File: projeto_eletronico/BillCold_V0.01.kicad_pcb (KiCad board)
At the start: 2 copper layers, 53 x 53 mm, 54 parts, among them J1 USB_B, SW1 SW_Push, SW2 SW_SPDT_321, U1 ESP32-S3, U2 AMS1117, U3 W25Q128JVSIQ, U4 USBLC6-2SC6, X1 OSCILADOR-3225

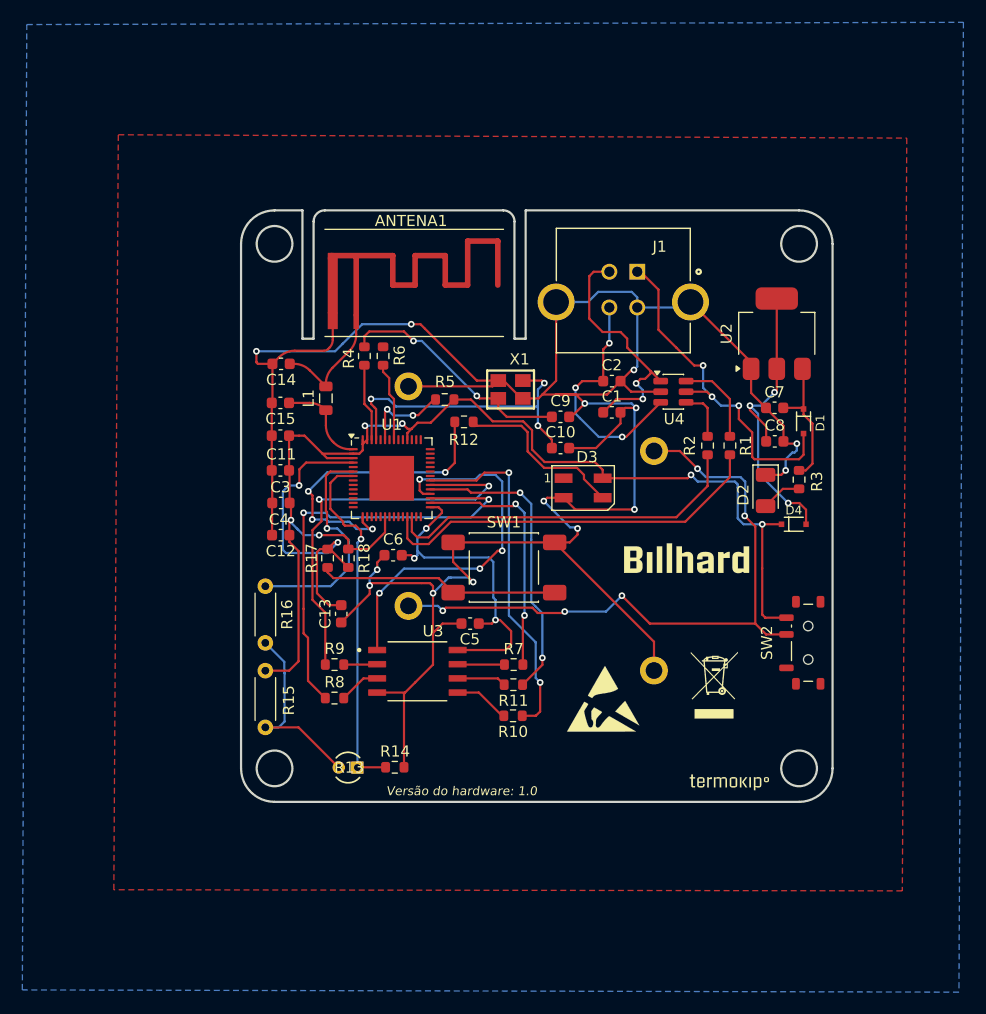
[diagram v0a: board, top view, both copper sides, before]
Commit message: Conclusão do projeto
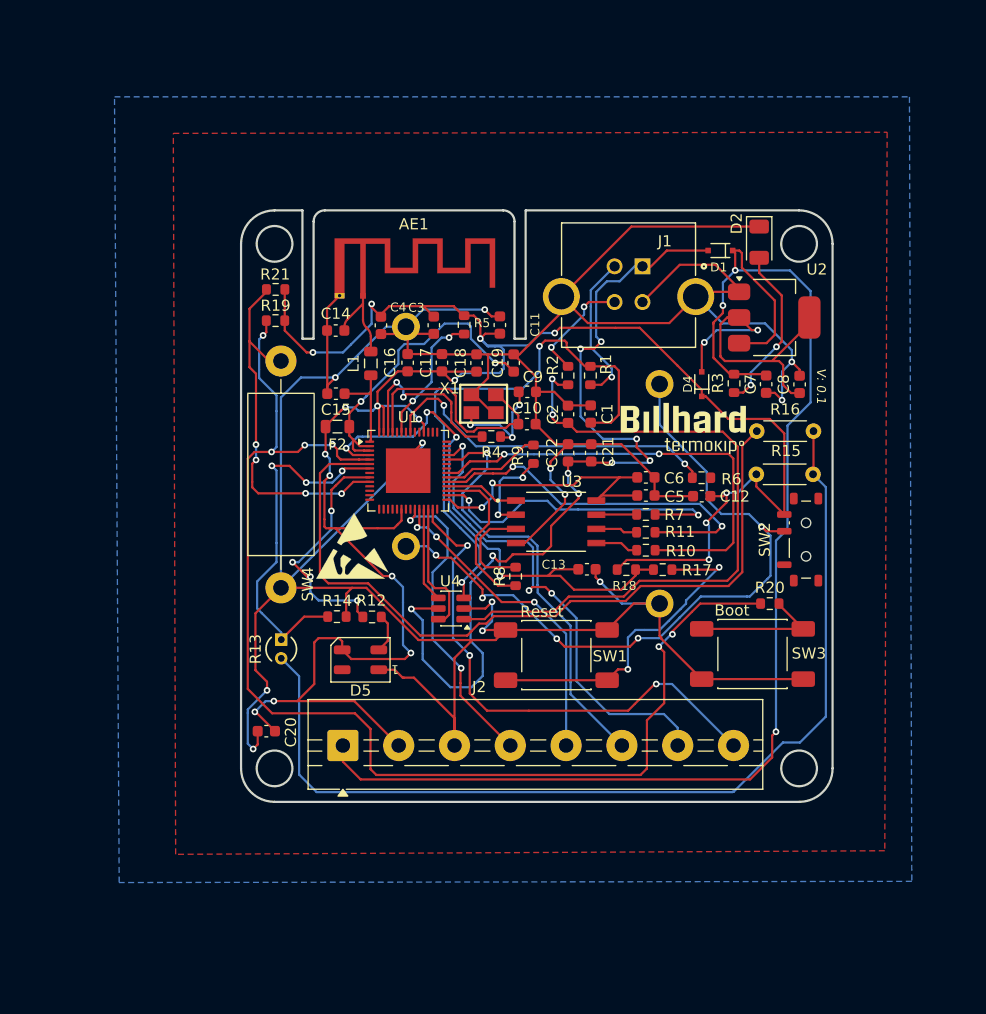
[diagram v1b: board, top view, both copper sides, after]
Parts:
- removed ANTENA1: ANT_2.4GB, ANTENA_2.4GZ:Antena_2.4GB
- removed D3: SK6812MINI, LED_SMD:LED_SK6812MINI_PLCC4_3.5x3.5mm_P1.75mm
- removed the REF** at (178.4, 119.0)
- added AE1: Antenna_Shield, RF_Antenna:Texas_SWRA117D_2.4GHz_Right, F.Cu at (146.9, 84.2)
- added C16: 10u, Capacitor_SMD:C_0603_1608Metric, F.Cu at (150.9, 90.2)
- added C17: 1u, Capacitor_SMD:C_0603_1608Metric, F.Cu at (154.0, 90.2)
- added C18: 100n, Capacitor_SMD:C_0603_1608Metric, F.Cu at (157.1, 90.2)
- added C19: 100n, Capacitor_SMD:C_0603_1608Metric, F.Cu at (160.4, 90.2)
- added C20: 100n, Capacitor_SMD:C_0603_1608Metric, F.Cu at (138.3, 123.2)
- added C21: 100n, Capacitor_SMD:C_0603_1608Metric, F.Cu at (167.4, 98.2)
- added C22: 4.7u, Capacitor_SMD:C_0603_1608Metric, F.Cu at (165.3, 98.2)
- added D5: SK6812, LED_SMD:LED_WS2812B-Mini_PLCC4_3.5x3.5mm, F.Cu at (146.7, 116.8)
- added F2: 600Ω, Inductor_SMD:L_0805_2012Metric, F.Cu at (144.6, 95.9)
- added J2: Screw_Terminal_01x08, TerminalBlock:TerminalBlock_MaiXu_MX126-5.0-08P_1x08_P5.00mm, F.Cu at (145.1, 124.5)
- added R19: 10k, Resistor_SMD:R_0603_1608Metric, F.Cu at (139.1, 86.4)
- added R20: 470, Resistor_SMD:R_0603_1608Metric, F.Cu at (183.4, 111.7)
- added R21: 10K, Resistor_SMD:R_0603_1608Metric, F.Cu at (139.1, 83.6)
- added SW3: SW_Push, Button_Switch_SMD:SW_Push_1P1T_NO_E-Switch_TL3301NxxxxxG, F.Cu at (181.8, 116.2)
- added SW4: SW_Reed, Resistor_THT:R_Axial_DIN0614_L14.3mm_D5.7mm_P20.32mm_Horizontal, F.Cu at (139.6, 110.3)
- C1, C2: value 1pF -> NC
- C11: value 0.1uF -> 1.1uF
- C12: value 0.1uF -> 100nF
- C3: value 10uF -> 1u
- C4: value 1uF -> 100nF
- C5: value 0.1uF -> 100n
- R1, R2: value 0h -> 0Ω
- R10, R11, R17, R4, R7, R8, R9: value 0 -> 0Ω
- R12: value 0 -> 360
- R6: value 499 -> 33
- moved R16 52.7 mm to (187.3, 96.3), turned to 180 degrees
- moved R15 47.4 mm to (182.2, 100.2), turned to 0 degrees
- moved C12 37.9 mm to (177.3, 102.1)
- moved R6 30.5 mm to (177.3, 100.5), turned to 0 degrees
- moved G*** 30.2 mm to (177.5, 97.6)
- moved R17 30.0 mm to (173.8, 108.7), turned to 180 degrees
- moved U4 27.8 mm to (154.8, 112.2), turned to 180 degrees
- moved REF** 26.3 mm to (146.0, 106.6)
- moved R9 25.9 mm to (162.2, 98.3), turned to -90 degrees
- moved R18 24.9 mm to (170.5, 108.7), turned to 0 degrees
- moved C6 23.7 mm to (172.3, 100.4), turned to 180 degrees
- moved C13 22.4 mm to (167.0, 108.7), turned to 180 degrees
- moved D2 22.3 mm to (182.4, 79.3)
- moved C11 22.0 mm to (159.2, 86.8), turned to 90 degrees
- moved R8 19.5 mm to (160.6, 109.3), turned to 90 degrees
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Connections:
- C1 pad 1: /D_N -> Net-(C1-Pad1)
- C2 pad 1: /D_P -> Net-(C2-Pad1)
- J1 pad 2: /D_N -> Net-(J1-D-)
- J1 pad 3: /D_P -> Net-(J1-D+)
- R1 pad 1: Net-(R1-Pad1) -> Net-(C1-Pad1)
- R1 pad 2: /D- -> Net-(J1-D-)
- R2 pad 1: Net-(R2-Pad1) -> Net-(J1-D+)
- R2 pad 2: /D+ -> Net-(C2-Pad1)
- U1 pad 10: unconnected-(U1-GPIO5-Pad10) -> /GPIO5
- U1 pad 15: /DATA_LED -> unconnected-(U1-GPIO10-Pad15)
- U1 pad 2: /VDD33 -> /VDD3P3
- U1 pad 23: unconnected-(U1-GPIO17-Pad23) -> /TX_LORA
- U1 pad 24: unconnected-(U1-GPIO18-Pad24) -> /RX_LORA
- U1 pad 27: unconnected-(U1-GPIO21-Pad27) -> /AU_LORA
- U1 pad 3: /VDD33 -> /VDD3P3
- U1 pad 38: unconnected-(U1-GPIO33-Pad38) -> /M0_LORA
- U1 pad 39: unconnected-(U1-GPIO34-Pad39) -> /M1_LORA
- U1 pad 5: unconnected-(U1-GPIO0-Pad5) -> /BOOT
- U1 pad 57: unconnected-(U1-GND-Pad57) -> GND
- U1 pad 9: unconnected-(U1-GPIO4-Pad9) -> /DATA_LED
- U4 pad 1: /D_N -> Net-(C2-Pad1)
- U4 pad 3: /D_P -> Net-(C1-Pad1)
- U4 pad 4: Net-(R2-Pad1) -> /D-
- U4 pad 6: Net-(R1-Pad1) -> /D+
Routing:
- net /BOOT: track 0.00 -> 109.8 mm, vias 0 -> 6
- net /VIN_5V: track 12.2 -> 121.0 mm, vias 0 -> 3
- net /VDD33: track 107.6 -> 199.8 mm, vias 6 -> 17
- net GND: track 238.9 -> 327.3 mm, vias 14 -> 12
- net Net-(R13-Pad2): track 17.8 -> 87.8 mm
- net Net-(C2-Pad1): track 0.00 -> 60.3 mm, vias 0 -> 2
- net Net-(J1-VBUS): track 31.7 -> 81.6 mm, vias 3 -> 9
- net /GPIO1: track 20.4 -> 69.5 mm, vias 1 -> 0
- net Net-(C1-Pad1): track 0.00 -> 48.2 mm, vias 0 -> 2
- net /AU_LORA: track 0.00 -> 47.1 mm, vias 0 -> 3
- net /M1_LORA: track 0.00 -> 43.8 mm, vias 0 -> 3
- net /M0_LORA: track 0.00 -> 39.0 mm, vias 0 -> 1
- net /GPIO5: track 0.00 -> 33.5 mm, vias 0 -> 4
- net /RX_LORA: track 0.00 -> 29.0 mm, vias 0 -> 3
- net /TX_LORA: track 0.00 -> 28.0 mm, vias 0 -> 2
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- added copper zone on B.Cu, net (none)
- added copper zone on F.Cu, net (none)
- removed copper zone on B.Cu, net GND
- removed copper zone on F.Cu, net GND
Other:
- board text added: "3.3V"
- board text added: "5V"
- board text added: "Boot"
- board text added: "GND"
- board text added: "IO17"
- board text added: "IO18"
- board text added: "IO21"
- board text added: "IO33"
- board text added: "IO34"
- board text added: "Reset"
- board text added: "V: 0.1"
- board text removed: "Versão do hardware: 1.0"
